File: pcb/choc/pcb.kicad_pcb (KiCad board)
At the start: 2 copper layers, 154.2 x 86 mm, 70 parts, among them J1 MJ-4PP-9, J2 USB_C_Receptacle_USB2.0, J3 Conn_01x04_Female, J4 Conn_01x08_Female, SW1 SW_PUSH, SW10 SW_PUSH, SW11 SW_PUSH, SW12 SW_PUSH, SW13 SW_PUSH, SW14 SW_PUSH, SW15 SW_PUSH, SW16 SW_PUSH, SW17 SW_PUSH, SW18 SW_PUSH, SW19 SW_PUSH, SW2 SW_PUSH, SW3 SW_PUSH, SW4 SW_PUSH, SW5 SW_PUSH, SW6 SW_PUSH, SW7 SW_PUSH, SW8 SW_PUSH, SW9 SW_PUSH, U1 rp2040-zero, U2 rp2040-zero, U3 roller

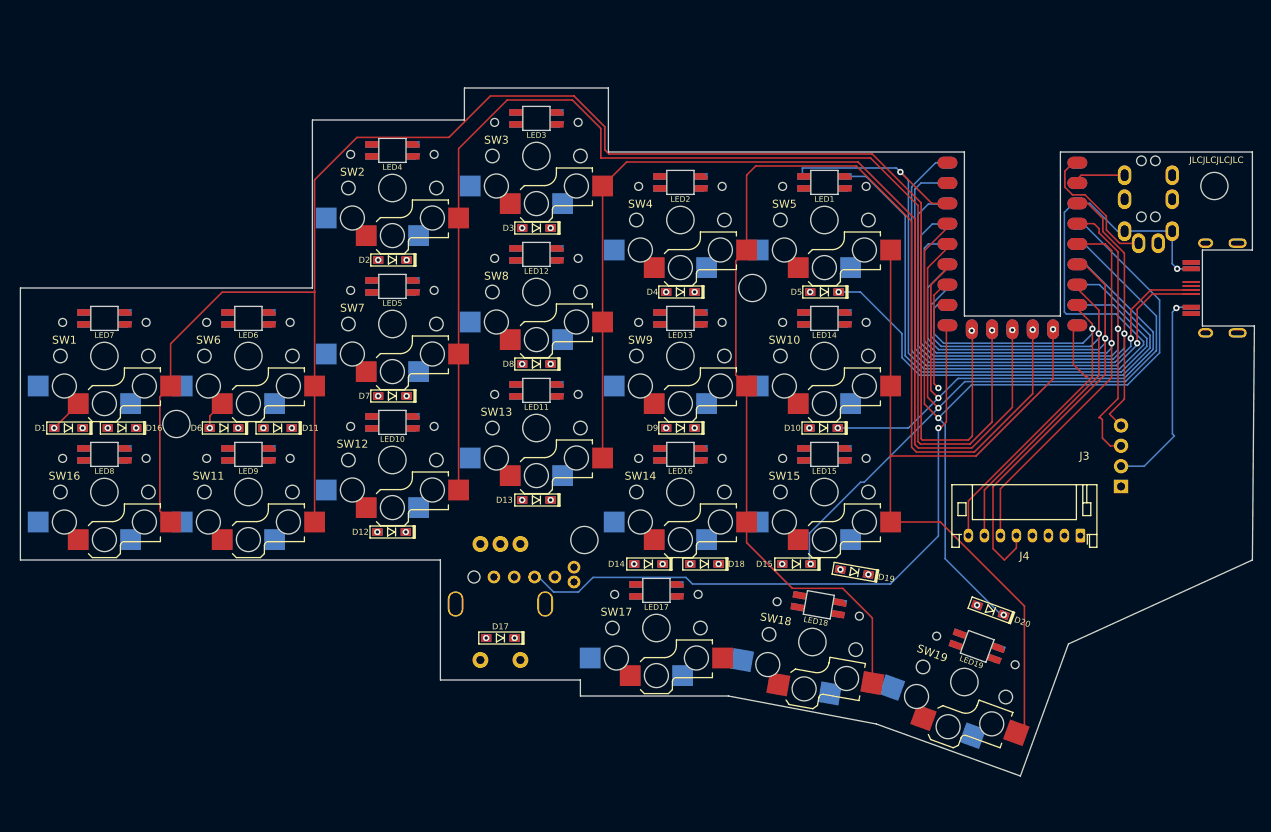
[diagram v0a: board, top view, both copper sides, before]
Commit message: prototype 0
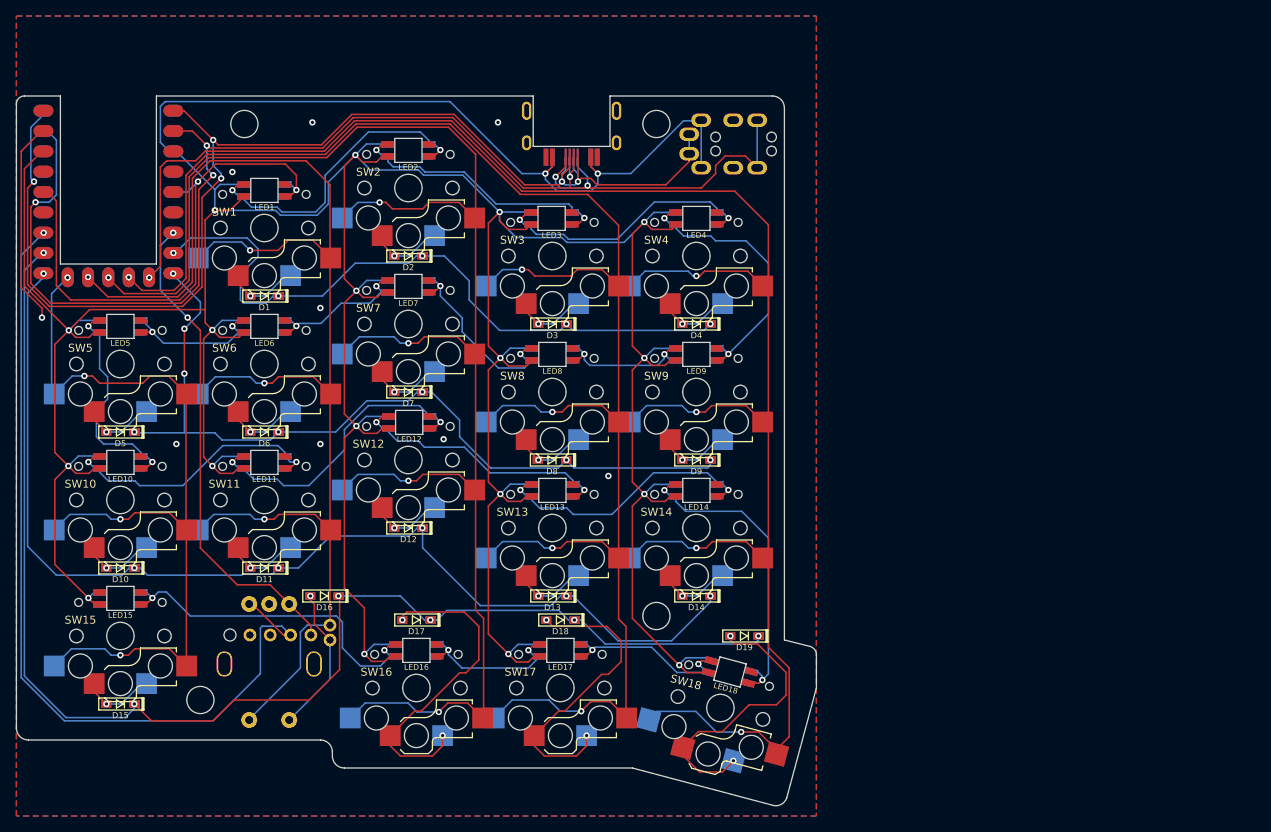
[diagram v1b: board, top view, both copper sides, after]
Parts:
- removed D20: D_Small, zzkeeb:Diode_1N4148-SOD123-reversible
- removed J3: Conn_01x04_Female, zzkeeb:Pointing_Cirque-adapter
- removed J4: Conn_01x08_Female, Connector_JST:JST_PH_S8B-PH-K_1x08_P2.00mm_Horizontal
- removed LED19: YS-SK6812MINI-E, zzkeeb:LED_SK6812-MINI-E-reversible
- removed SW19: SW_PUSH, zzkeeb:Switch_ChocV1-hotswap-reversible
- D1, D10, D11, D12, D13, D14, D15, D16, D17, D18, D19, D2, D3, D4, D5, D6, D7, D8, D9: moved to B.Cu
- J1: value MJ-4PP-9 -> AudioJack4
- LED1, LED10, LED11, LED12, LED13, LED14, LED15, LED16, LED17, LED18, LED2, LED3, LED4, LED5, LED6, LED7, LED8, LED9: value YS-SK6812MINI-E -> LED_SK6812MINI-E
- SW1, SW10, SW11, SW12, SW13, SW14, SW15, SW16, SW17, SW18, SW2, SW3, SW4, SW5, SW6, SW7, SW8, SW9: value SW_PUSH -> Switch
- U1, U2: value rp2040-zero -> MCU_rp2040-zero
- U3: value roller -> RollerEncoder_EVQWGD001
- moved U1 113.2 mm to (64.0, 52.5)
- moved U2 113.2 mm to (64.0, 52.5)
- moved LED15 89.8 mm to (65.5, 103.3)
- moved SW10 89.8 mm to (65.5, 91.0)
- moved SW15 89.8 mm to (65.5, 108.0)
- moved SW5 89.8 mm to (65.5, 74.0)
- moved D5 89.7 mm to (65.5, 82.5)
- moved D10 89.6 mm to (65.5, 99.5)
- moved D15 86.3 mm to (65.5, 116.5)
- moved J2 82.9 mm to (121.9, 45.0), turned to 180 degrees
- moved H1 70.2 mm to (132.5, 44.0)
- moved LED1 70.0 mm to (83.5, 52.3)
- moved H4 66.7 mm to (81.0, 44.0)
- moved LED8 57.4 mm to (119.5, 72.8)
- moved LED9 57.4 mm to (137.5, 72.8)
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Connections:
- D10 pad 1: row1 -> row2
- D15 pad 1: row2 -> row3
- D16 pad 2: Net-(D16-Pad2) -> SW_ENCA
- D17 pad 2: SW_ENCA -> Net-(D17-Pad2)
- D5 pad 1: row0 -> row1
- LED15 pad 2: Net-(LED15-Pad2) -> unconnected-(LED15-Pad2)
- LED15 pad 4: Net-(LED14-Pad2) -> Net-(LED15-Pad4)
- LED16 pad 2: Net-(LED16-Pad2) -> Net-(LED15-Pad4)
- LED16 pad 4: Net-(LED15-Pad2) -> Net-(LED16-Pad4)
- LED17 pad 2: Net-(LED17-Pad2) -> Net-(LED16-Pad4)
- LED17 pad 4: Net-(LED16-Pad2) -> Net-(LED17-Pad4)
- LED18 pad 2: Net-(LED18-Pad2) -> Net-(LED17-Pad4)
- LED18 pad 4: Net-(LED17-Pad2) -> Net-(LED14-Pad2)
- LED5 pad 2: Net-(LED5-Pad2) -> Net-(LED10-Pad4)
- LED5 pad 4: Net-(LED4-Pad2) -> Net-(LED5-Pad4)
- LED6 pad 2: Net-(LED6-Pad2) -> Net-(LED5-Pad4)
- LED6 pad 4: Net-(LED5-Pad2) -> Net-(LED6-Pad4)
- LED7 pad 2: Net-(LED7-Pad2) -> Net-(LED6-Pad4)
- LED7 pad 4: Net-(LED6-Pad2) -> Net-(LED7-Pad4)
- LED8 pad 2: Net-(LED8-Pad2) -> Net-(LED7-Pad4)
- LED8 pad 4: Net-(LED7-Pad2) -> Net-(LED8-Pad4)
- LED9 pad 2: Net-(LED10-Pad4) -> Net-(LED8-Pad4)
- LED9 pad 4: Net-(LED8-Pad2) -> Net-(LED4-Pad2)
- SW1 pad 2: col0 -> col1
- SW10 pad 2: col4 -> col0
- SW11 pad 2: col0 -> col1
- SW12 pad 2: col1 -> col2
- SW13 pad 2: col2 -> col3
- SW14 pad 2: col3 -> col4
- SW15 pad 2: col4 -> col0
- SW16 pad 1: Net-(D16-Pad2) -> Net-(D17-Pad2)
- SW16 pad 2: col0 -> col2
- SW17 pad 2: col2 -> col3
- SW18 pad 2: col3 -> col4
- SW2 pad 2: col1 -> col2
- SW3 pad 2: col2 -> col3
- SW4 pad 2: col3 -> col4
- SW5 pad 2: col4 -> col0
- SW6 pad 2: col0 -> col1
- SW7 pad 2: col1 -> col2
- SW8 pad 2: col2 -> col3
- SW9 pad 2: col3 -> col4
- U1 pad 15: ENCA -> row1
- U1 pad 16: LED -> row0
- U1 pad 17: row0 -> ENCA
- U1 pad 18: row1 -> unconnected-(U1-Pad18)
- U1 pad 19: row2 -> LED
- U1 pad 20: row3 -> unconnected-(U1-Pad20)
- U1 pad 3: SCLK/SDA -> unconnected-(U1-Pad3)
- U1 pad 4: MOSI/SCL -> unconnected-(U1-Pad4)
- U1 pad 5: MISO/DC -> unconnected-(U1-Pad5)
- U1 pad 6: CS -> unconnected-(U1-Pad6)
- U1 pad 7: RST -> ENCB
- U1 pad 8: BL -> row3
- U1 pad 9: ENCB -> row2
- U2 pad 15: ENCB -> row2
- U2 pad 16: LED -> row3
- U2 pad 17: row0 -> ENCB
- U2 pad 18: row1 -> unconnected-(U2-Pad18)
- U2 pad 19: row2 -> LED
- U2 pad 20: row3 -> unconnected-(U2-Pad20)
- U2 pad 3: SCLK/SDA -> unconnected-(U2-Pad3)
- U2 pad 4: MOSI/SCL -> unconnected-(U2-Pad4)
- U2 pad 5: MISO/DC -> unconnected-(U2-Pad5)
- U2 pad 6: CS -> unconnected-(U2-Pad6)
- U2 pad 7: RST -> ENCA
- U2 pad 8: BL -> row0
- U2 pad 9: ENCA -> row1
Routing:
- net VCC: track 148.9 -> 634.0 mm, vias 3 -> 20
- net col4: track 102.4 -> 243.2 mm, vias 1 -> 5
- net col0: track 224.3 -> 106.6 mm, vias 1 -> 4
- net RX: track 73.3 -> 170.7 mm, vias 1 -> 6
- net MISO/DC: track 86.6 -> 0.00 mm, vias 1 -> 0
- net CS: track 83.8 -> 0.00 mm, vias 1 -> 0
- net SCLK/SDA: track 82.9 -> 0.00 mm, vias 1 -> 0
- net col2: track 130.2 -> 211.8 mm, vias 1 -> 5
- net MOSI/SCL: track 80.7 -> 0.00 mm, vias 1 -> 0
- net TX: track 85.4 -> 157.4 mm, vias 1 -> 5
- net RST: track 68.7 -> 0.00 mm, vias 1 -> 0
- net col3: track 154.0 -> 222.0 mm, vias 1 -> 5
- net BL: track 63.1 -> 0.00 mm, vias 1 -> 0
- net row3: track 106.9 -> 166.0 mm
- net ENCA: track 7.54 -> 61.1 mm, vias 0 -> 2
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- added copper zone on B.Cu, net GND
- added copper zone on F.Cu, net GND
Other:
- board size 154.2 x 86 mm -> 100 x 88.7 mm
- board text removed: "JLCJLCJLCJLC"
